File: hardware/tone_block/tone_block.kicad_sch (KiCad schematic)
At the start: 16 parts, among them J1 I/O, Q1 RS32716R

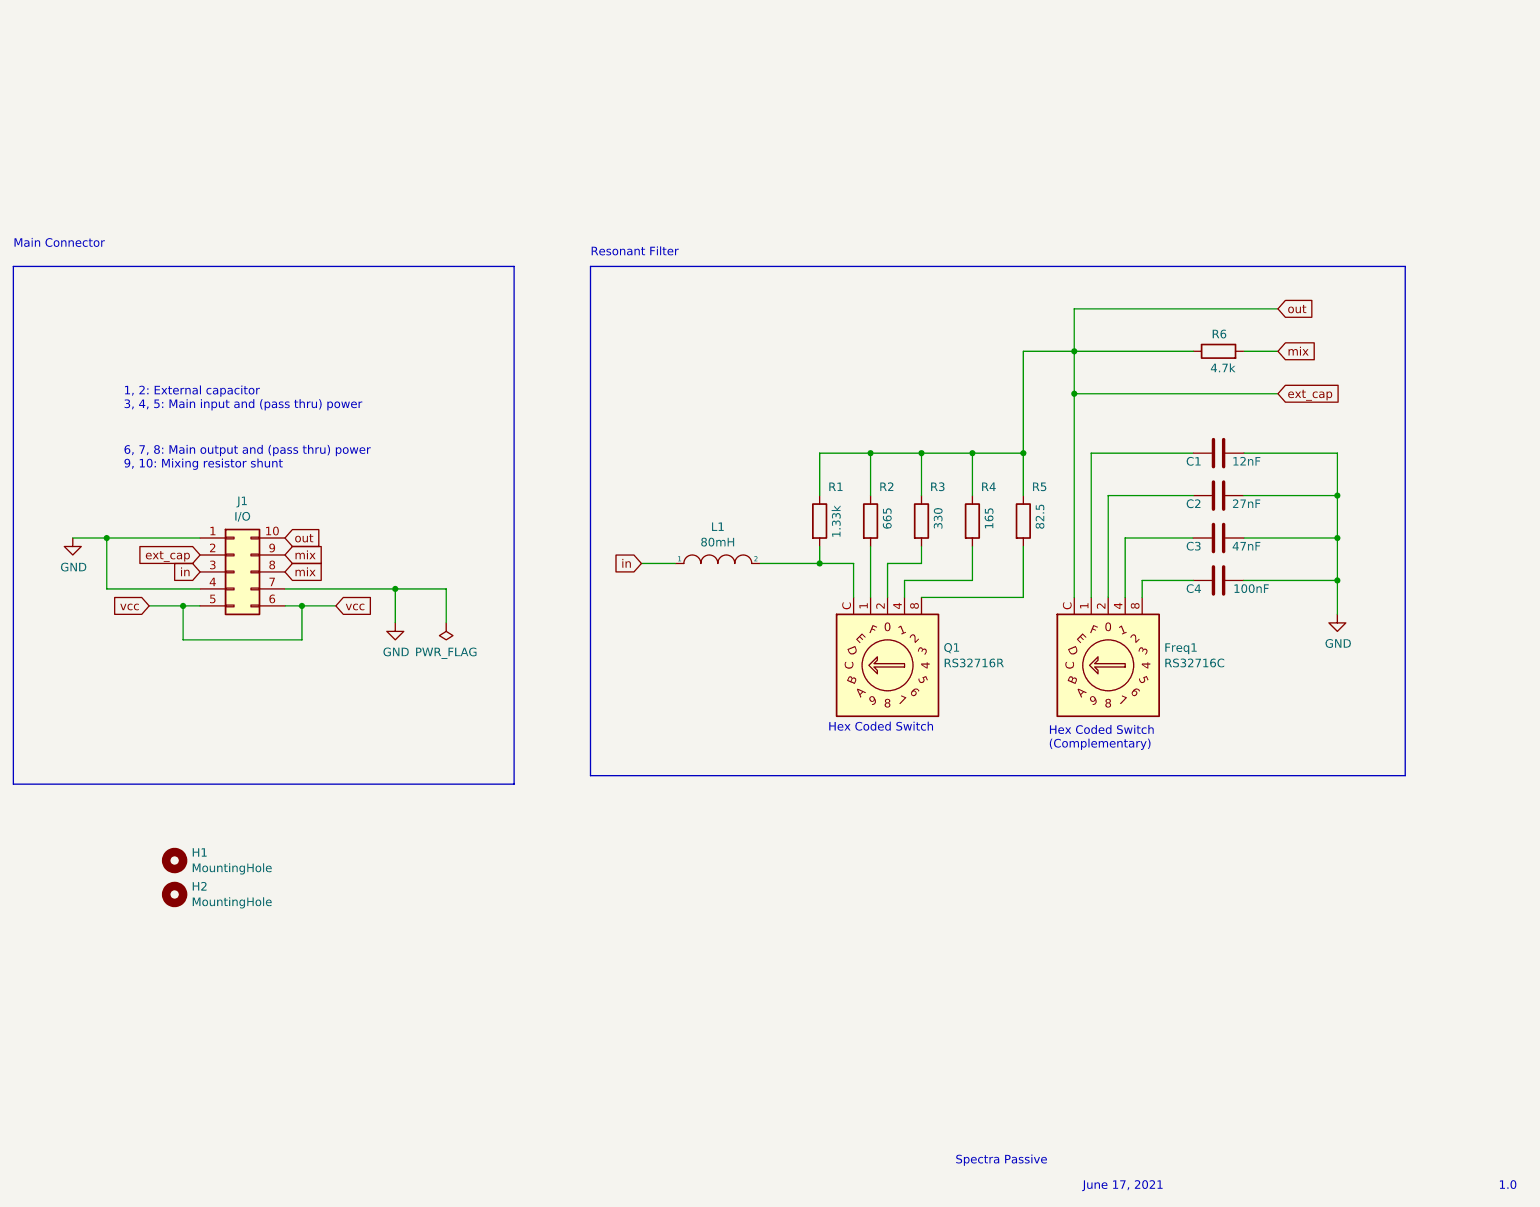
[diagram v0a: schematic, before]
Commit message: Tone block v2
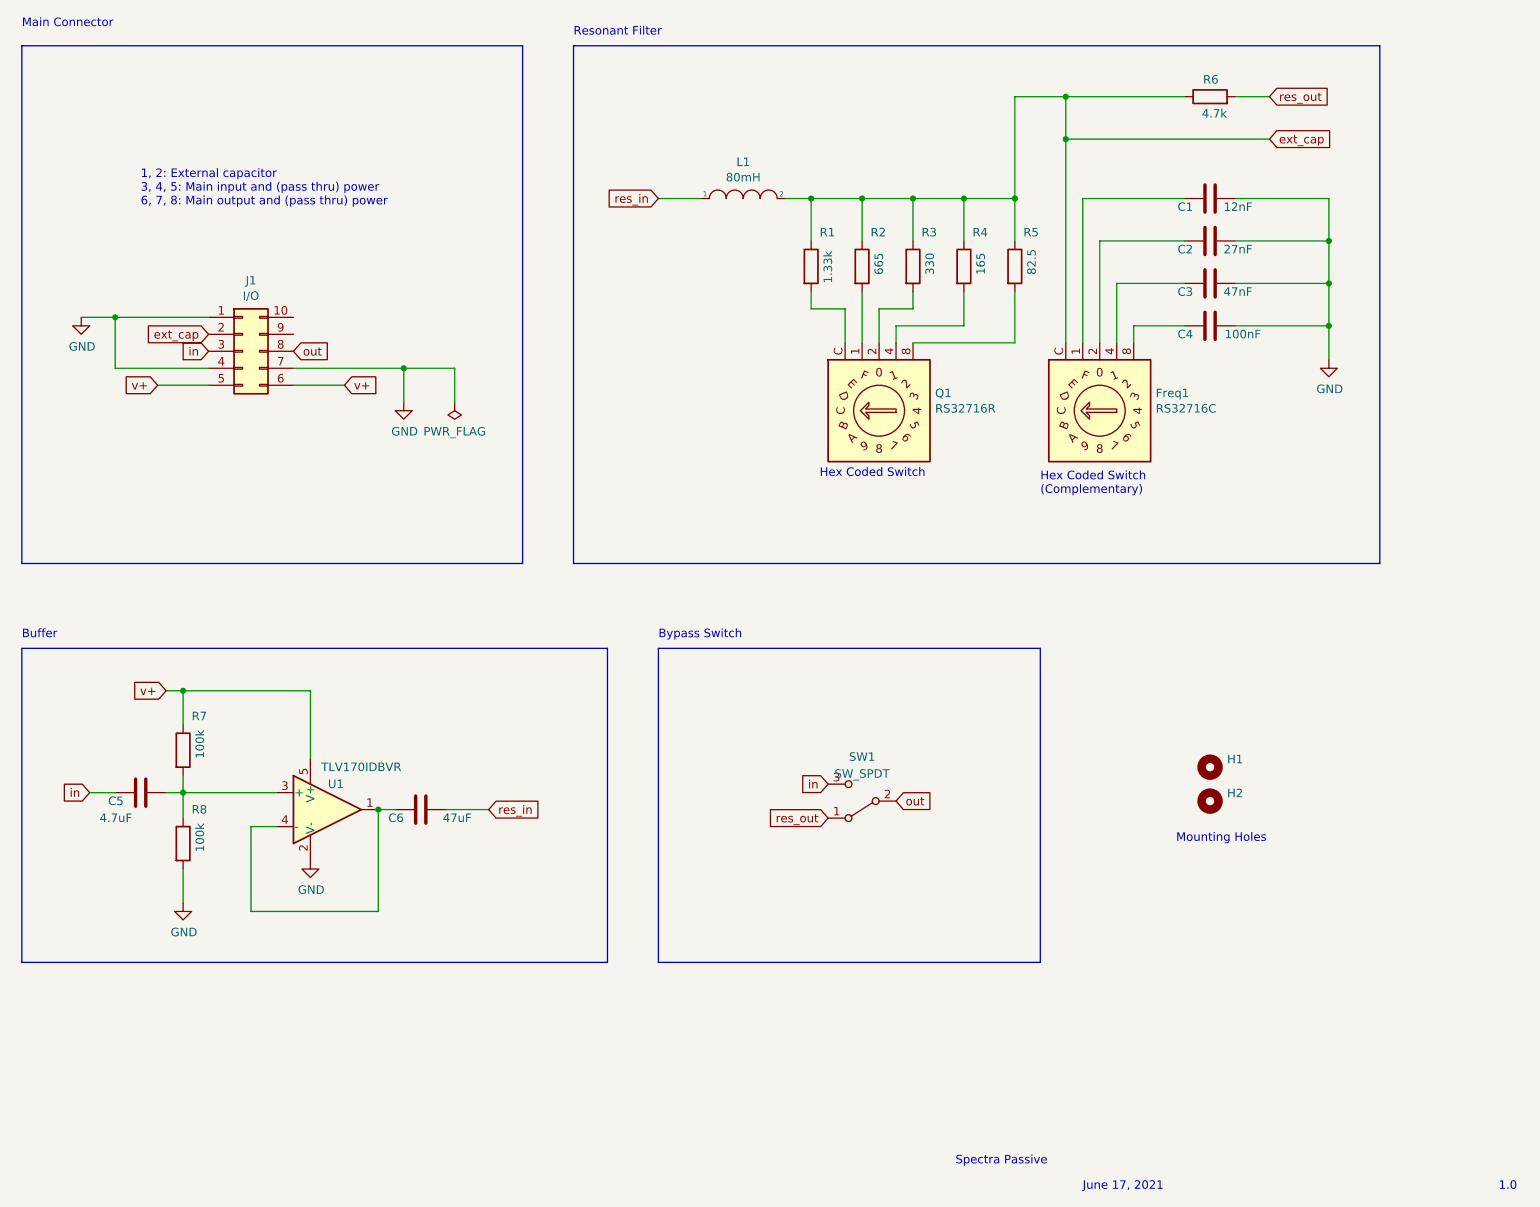
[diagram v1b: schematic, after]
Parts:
- added C5: 4.7uF, Capacitor_SMD:C_0603_1608Metric, symbol Device:C
- added C6: 47uF, Capacitor_SMD:C_0603_1608Metric, symbol Device:C
- added R7, R8: 100k, Resistor_SMD:R_0402_1005Metric, symbol Device:R
- added SW1: SW_SPDT, symbol Switch:SW_SPDT
- added U1: TLV170IDBVR, Package_TO_SOT_SMD:SOT-23-5, symbol cycfi_library:opamp_dbv
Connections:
- net GND: now also R8.2, U1.2 (V-)
- net ext_cap: now also L1.2; no longer J1.10 (Pin_10)
- net in: now also C5.2, SW1.3 (C); no longer L1.1
- net at Q1.C, R1.2: no longer L1.2
- removed net mix: J1.8 (Pin_8), J1.9 (Pin_9), R6.2
- net vcc renamed v+
- net v+: now also R7.1, U1.5 (V+)
- new net: C6.2, U1.1, U1.4 (-)
- new net: C5.1, R7.2, R8.1, U1.3 (+)
- new net out: J1.8 (Pin_8), SW1.2 (B)
- new net res_in: C6.1, L1.1
- new net res_out: R6.2, SW1.1 (A)
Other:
- note added: "1, 2: External capacitor 3, 4, 5: Main input and (pass thru) power 6, 7, 8: Main output and (pass thru) power"
- note added: "Buffer"
- note added: "Bypass Switch"
- note added: "Mounting Holes"
- note removed: "1, 2: External capacitor 3, 4, 5: Main input and (pass thru) power"
- note removed: "6, 7, 8: Main output and (pass thru) power 9, 10: Mixing resistor shunt"
- moved on the sheet: C1, C2, C3, C4, Freq1, H1, H2, J1, L1, Q1, R1, R2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
